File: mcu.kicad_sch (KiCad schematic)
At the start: 20 parts, among them J1 Conn_01x02_Pin, J2 Conn_01x02_Pin, J4 Conn_02x08_Counter_Clockwise, J6 Conn_01x02_Pin, SW85 SW_Push, SW86 SW_Push, SW87 SW_Push, SW89 SW_Push, U1 ESP32-S3-WROOM-1

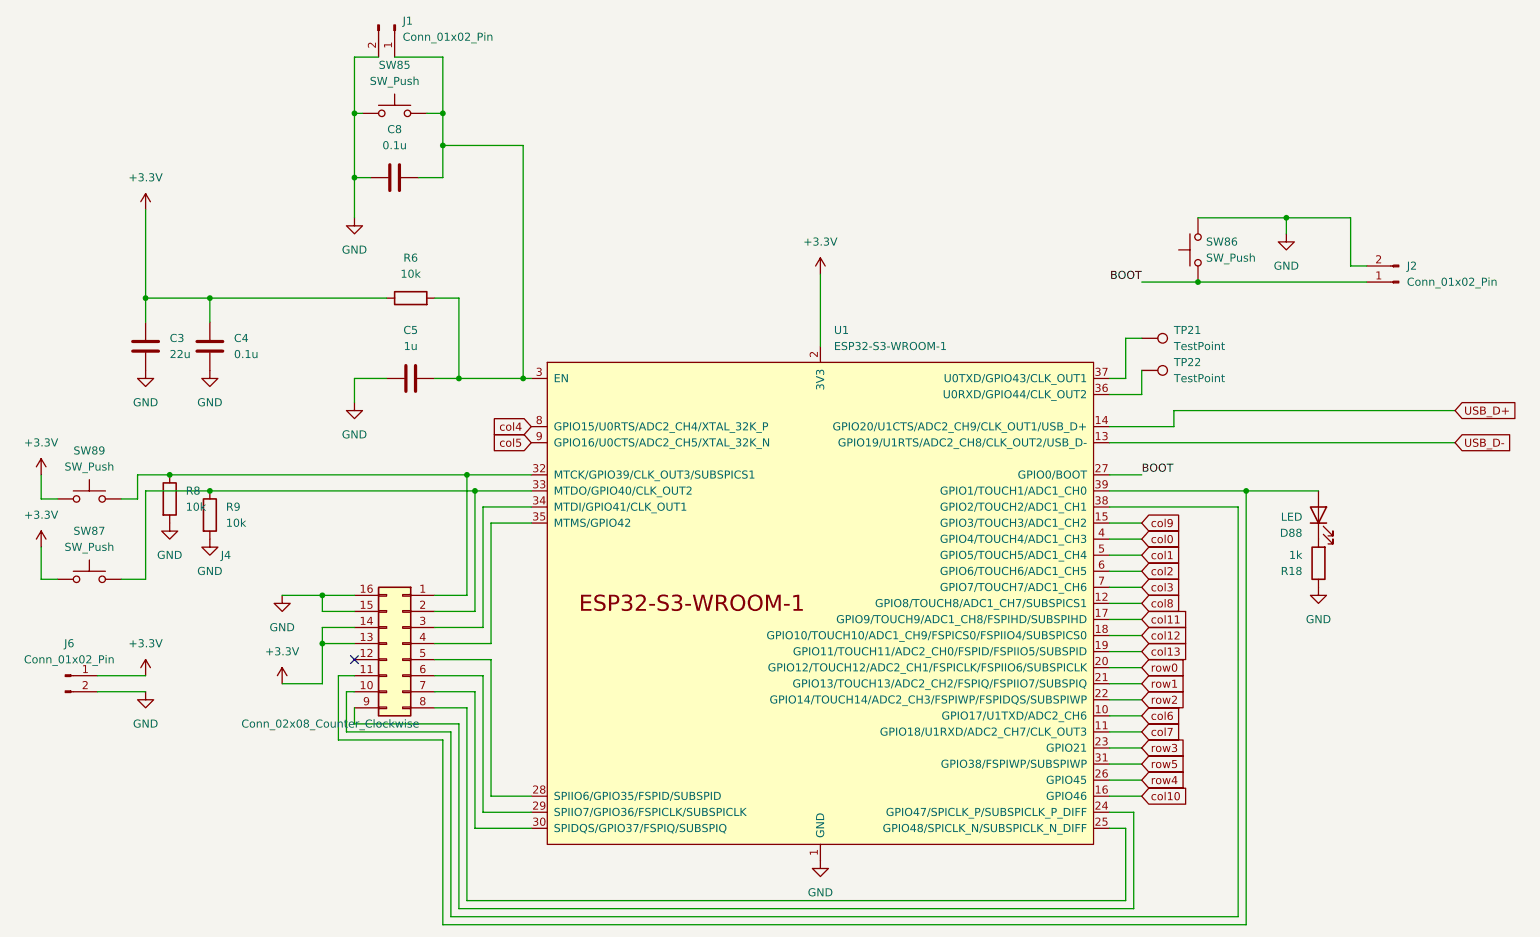
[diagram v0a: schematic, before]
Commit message: sent to fab
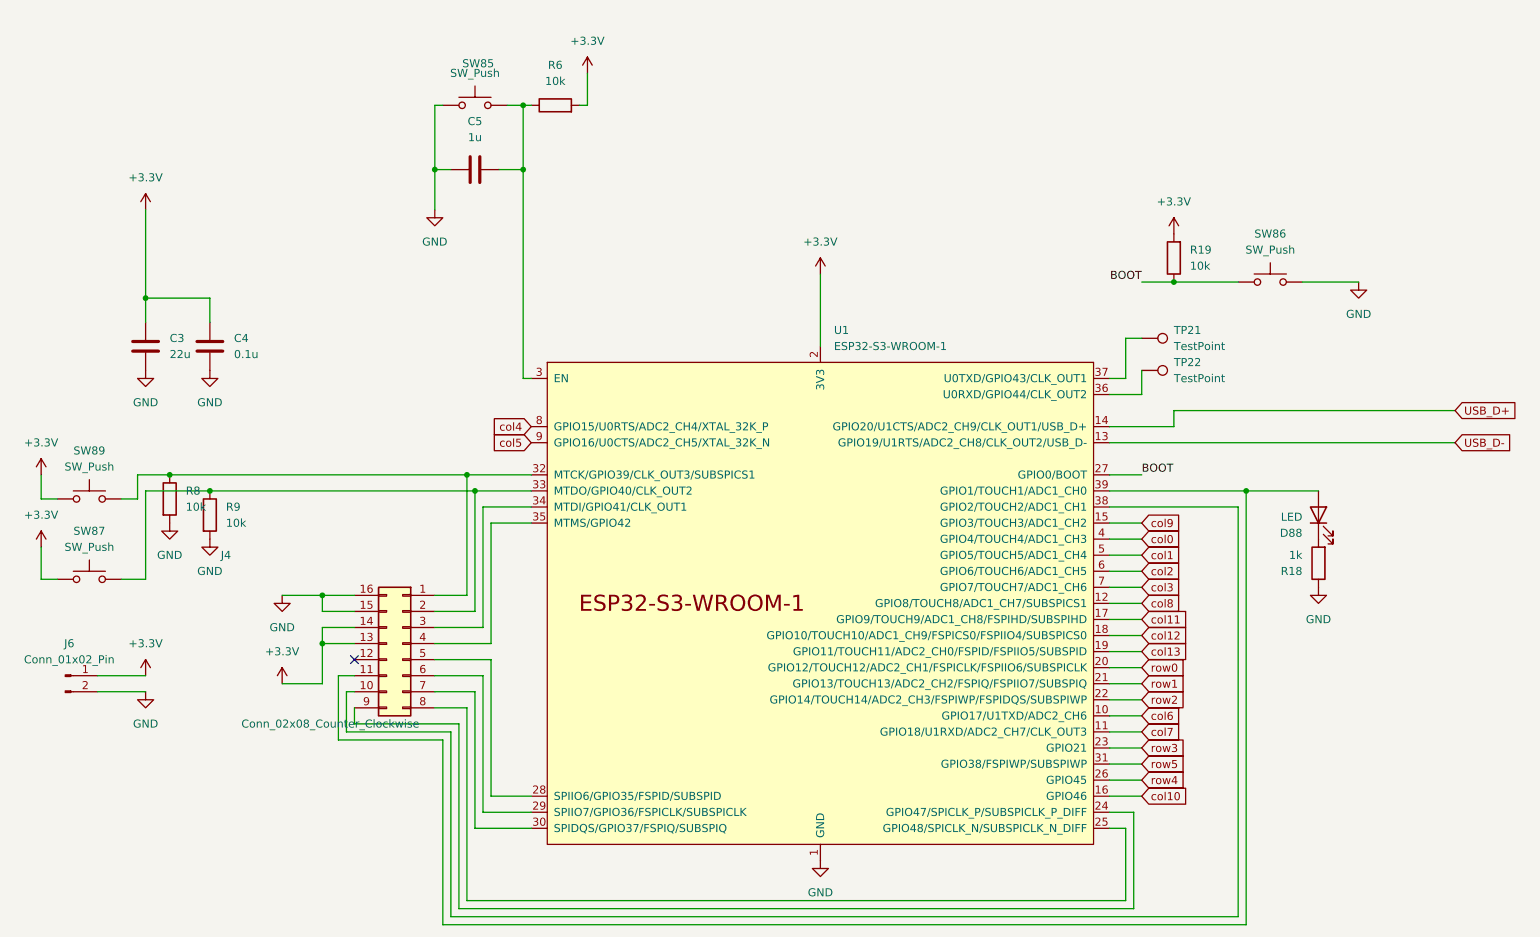
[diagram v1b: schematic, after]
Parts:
- removed C8: 0.1u, Capacitor_SMD:C_0805_2012Metric_Pad1.18x1.45mm_HandSolder, symbol Device:C
- removed J1, J2: Conn_01x02_Pin, Connector_PinHeader_2.54mm:PinHeader_1x02_P2.54mm_Vertical, symbol Connector:Conn_01x02_Pin
- added R19: 10k, Resistor_SMD:R_0805_2012Metric_Pad1.20x1.40mm_HandSolder, symbol Device:R
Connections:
- net +3.3V: now also R6.2, R19.2; no longer R6.1
- net BOOT: now also R19.1
- net at C5.2, SW85.2, U1.3 (EN): now also R6.1; no longer R6.2
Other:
- moved on the sheet: C5, R6, SW85, SW86
